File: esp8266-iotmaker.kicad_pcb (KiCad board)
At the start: 2 copper layers, 46 x 25.7 mm, 54 parts, among them J1 CONN_01X10, J2 CONN_01X10, Q1 S8050, Q2 S8050, SW1 SW_Push, SW2 SW_Push, U1 usb_mini_b, U2 chip-esp8266, U3 CP2102, U4 25Q32, U6 AMS1117-3.3, Y1 26MHz

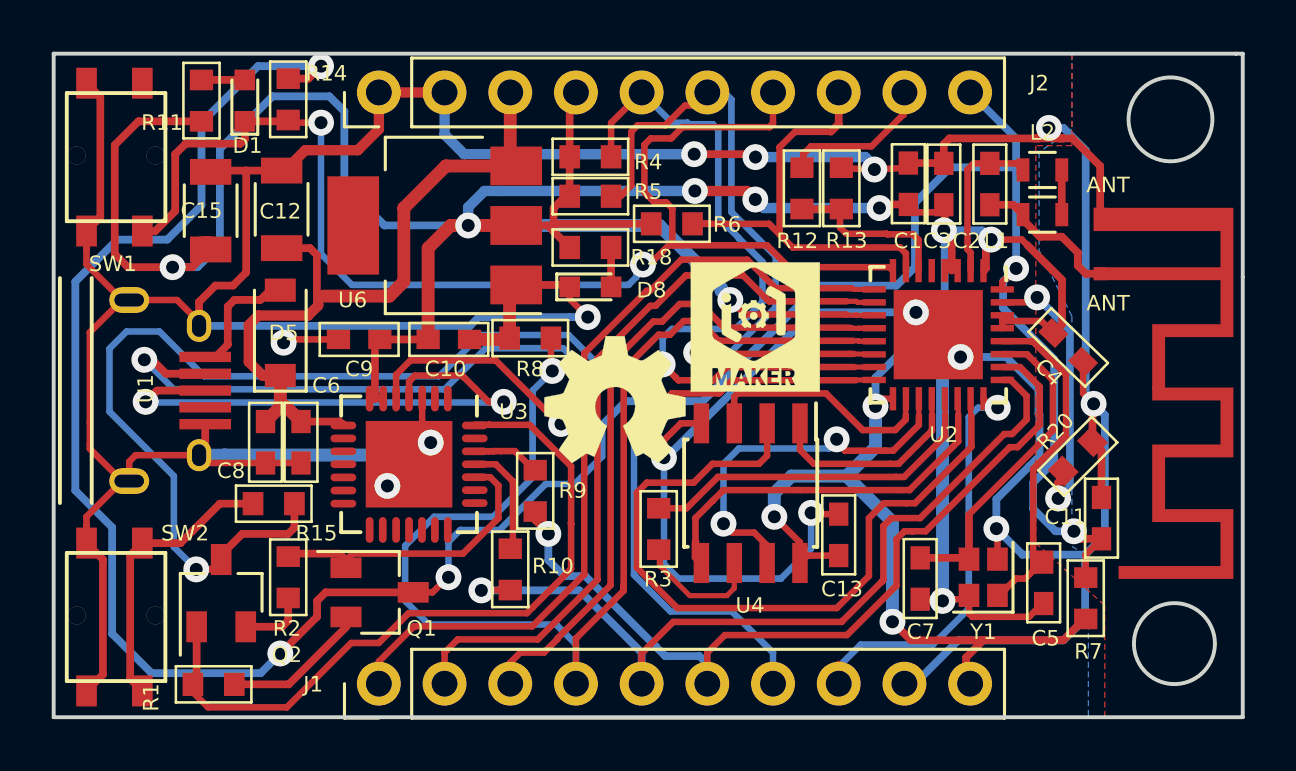
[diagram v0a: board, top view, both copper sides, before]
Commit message: edit solder mark
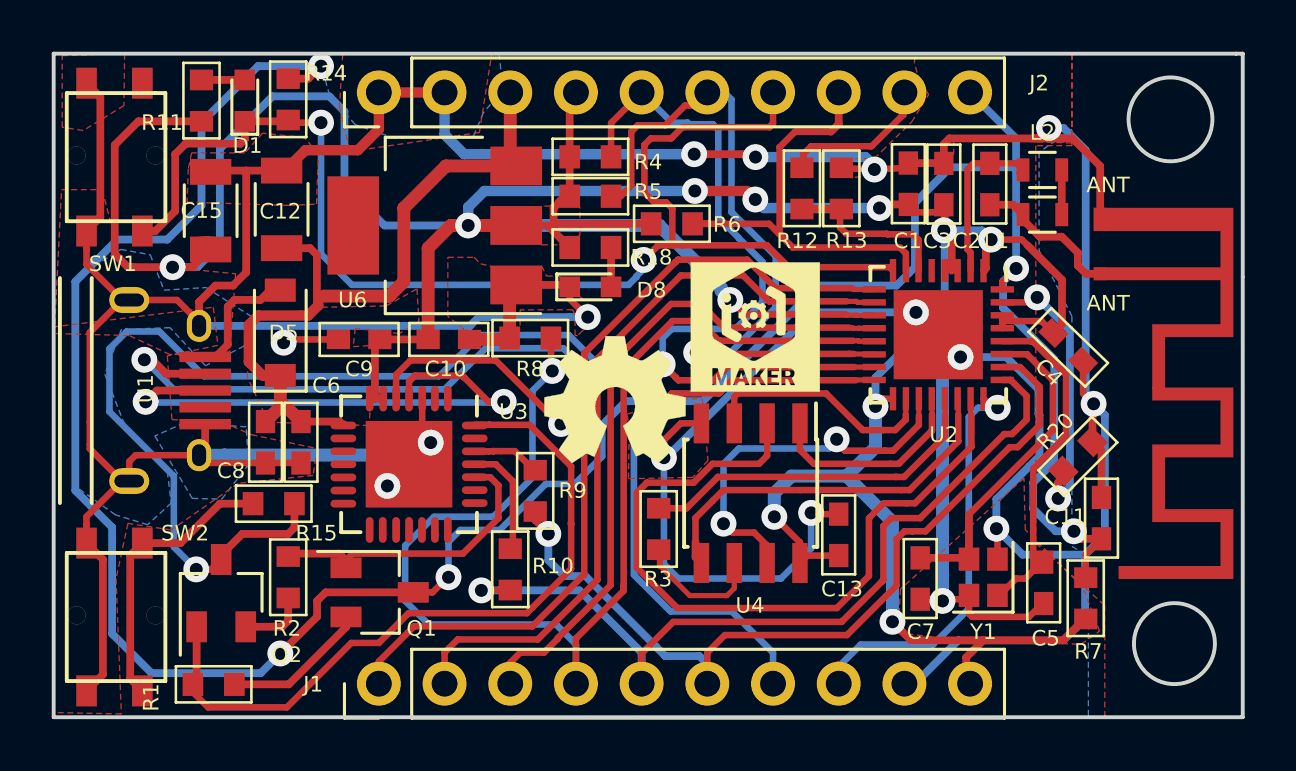
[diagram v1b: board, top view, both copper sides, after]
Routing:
- net GPIO14: track 32.4 -> 33.3 mm
- added copper zone on F.Cu, net 3V3

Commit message: edit pcb
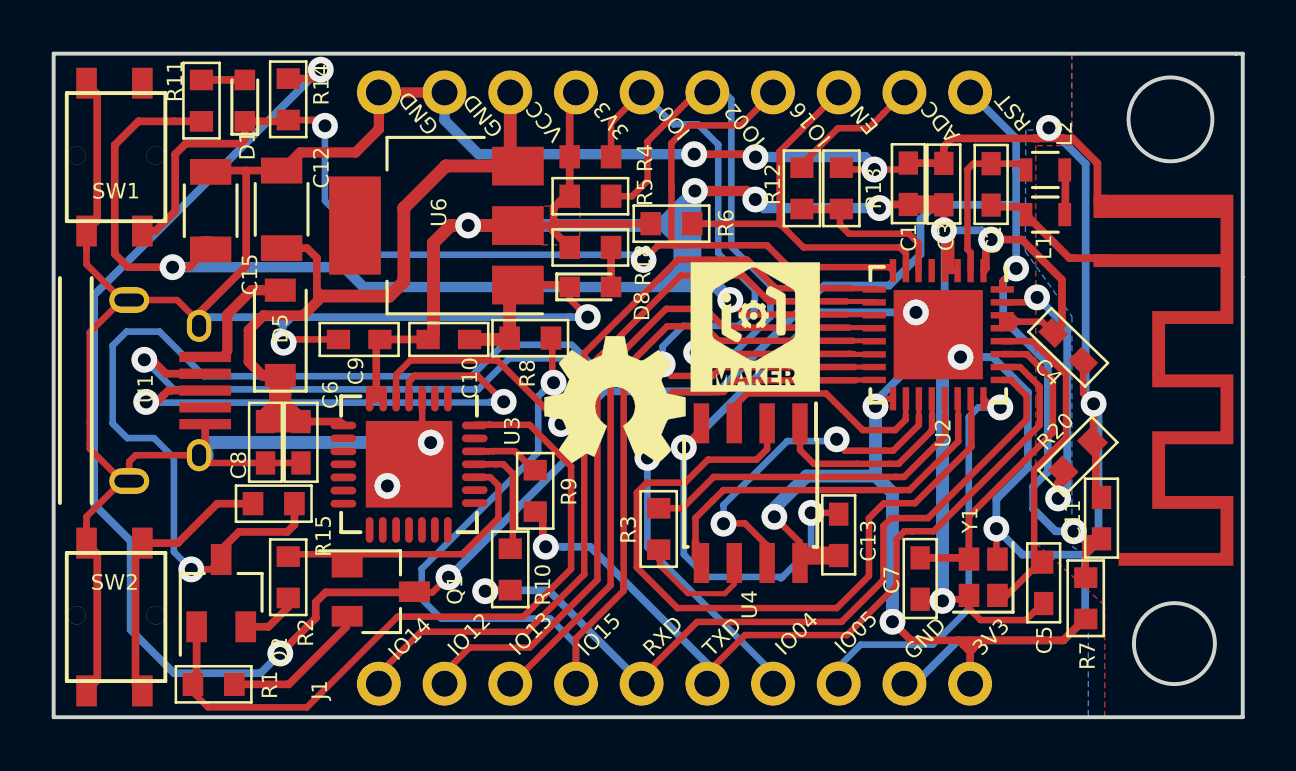
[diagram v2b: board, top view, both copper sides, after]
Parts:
- moved ANT 0.51 mm to (170.3, 94.4)
- moved L1 0.11 mm to (167.9, 95.1)
- moved L2 0.11 mm to (167.9, 93.4)
- moved U6 0.07 mm to (144.3, 95.5)
- moved Q1 0.05 mm to (142.2, 109.7)
- moved C2 0.05 mm to (165.8, 94.0)
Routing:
- net 3V3: track 146.2 -> 153.8 mm
- net GND: track 236.6 -> 231.6 mm
- net REST: track 101.6 -> 96.7 mm
- net GPIO16: track 50.8 -> 46.6 mm
- net GPIO2: track 30.0 -> 27.8 mm
- net GPIO15: track 46.6 -> 44.7 mm
- net GPIO4: track 23.5 -> 21.7 mm
- net RXD: track 32.7 -> 31.1 mm
- net VCC: track 28.4 -> 29.6 mm
- net EN: track 16.9 -> 15.7 mm
- net Net-(U6-Pad4): track 1.13 -> 0.00 mm
- net GPIO0: track 67.8 -> 66.9 mm
- net GPIO10: track 14.6 -> 13.6 mm
- net TXD: track 33.6 -> 32.9 mm
- net ADC_EX: track 5.99 -> 5.32 mm
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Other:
- net class Default: trace_width 0.2 -> 0.254
- board text added: "ADC"
- board text added: "EN"
- board text added: "IO0"
- board text added: "IO02"
- board text added: "IO04"
- board text added: "IO05"
- board text added: "IO12"
- board text added: "IO13"
- board text added: "IO14"
- board text added: "IO15"
- board text added: "IO16"
- board text added: "RST"
